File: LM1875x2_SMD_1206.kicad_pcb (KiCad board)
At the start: 2 copper layers, 27 parts, among them J1 INPUT, J2 OUTPUT, J3 POWER, U1 LM1875, U2 LM1875

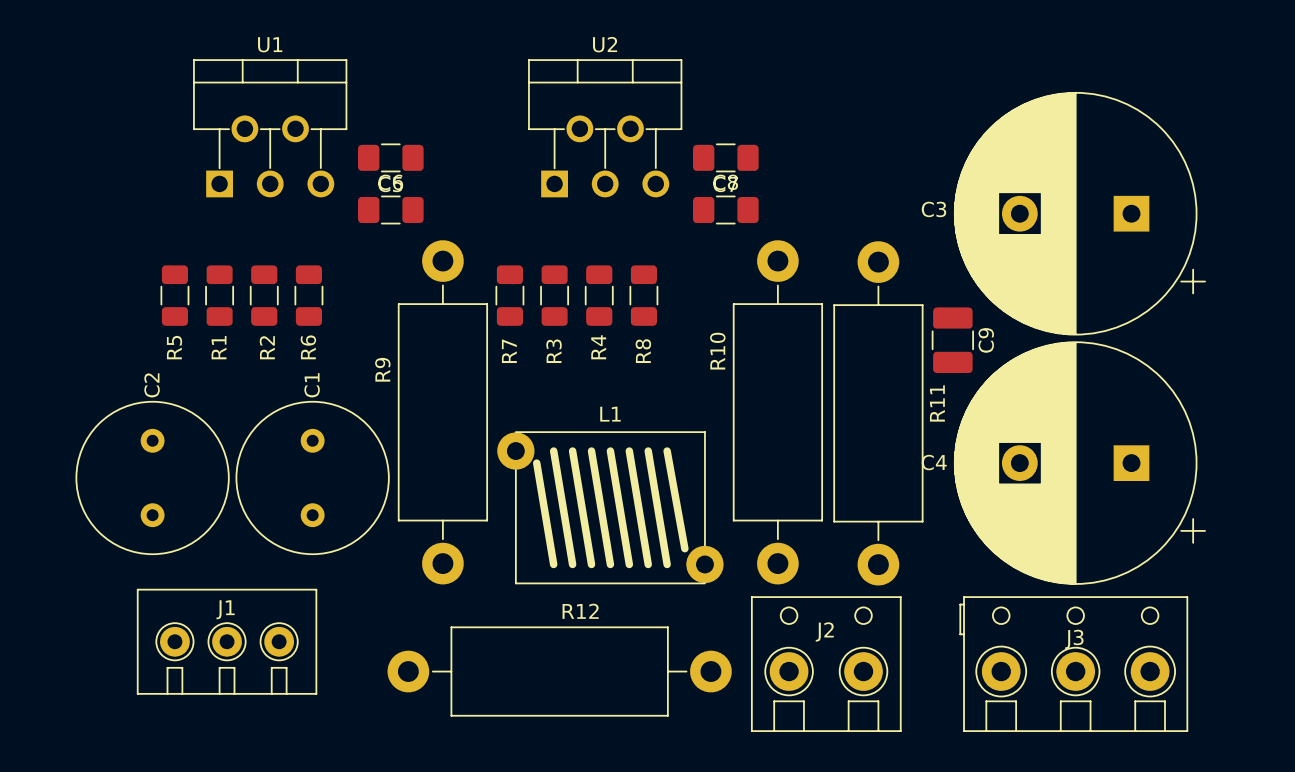
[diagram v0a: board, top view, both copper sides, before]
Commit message: finished layout
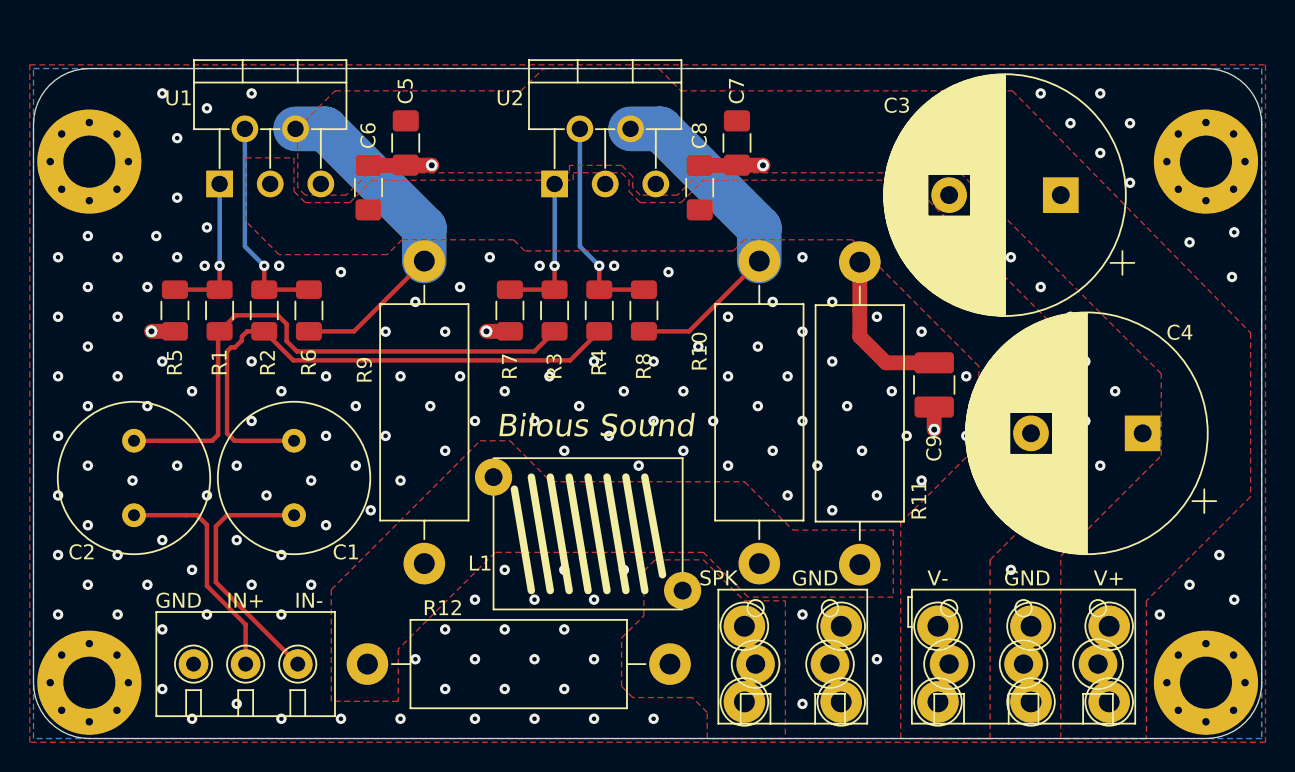
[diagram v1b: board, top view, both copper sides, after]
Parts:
- added H1: MountingHole, MountingHole:MountingHole_3.5mm_Pad_Via, F.Cu at (86.2, 88.8)
- added H2: MountingHole, MountingHole:MountingHole_3.5mm_Pad_Via, F.Cu at (86.2, 53.8)
- added H3: MountingHole, MountingHole:MountingHole_3.5mm_Pad_Via, F.Cu at (161.2, 53.8)
- added H4: MountingHole, MountingHole:MountingHole_3.5mm_Pad_Via, F.Cu at (161.2, 88.8)
- added J4: VCC, local_lib_footprints:Terminal_.25_PCB_TAB_TE_Connectivity_P5.08mm_, F.Cu at (154.8, 87.5)
- added J5: GND, local_lib_footprints:Terminal_.25_PCB_TAB_TE_Connectivity_P5.08mm_, F.Cu at (136.8, 87.5)
- added J6: VEE, local_lib_footprints:Terminal_.25_PCB_TAB_TE_Connectivity_P5.08mm_, F.Cu at (143.2, 87.5)
- added J7: SPK, local_lib_footprints:Terminal_.25_PCB_TAB_TE_Connectivity_P5.08mm_, F.Cu at (130.2, 87.5)
- added J8: GND, local_lib_footprints:Terminal_.25_PCB_TAB_TE_Connectivity_P5.08mm_, F.Cu at (149.5, 87.5)
- moved C3 4.91 mm to (151.5, 56.0)
- moved J3 3.54 mm to (149.0, 87.5)
- moved C9 3.25 mm to (143.0, 68.8)
- moved R12 2.80 mm to (125.2, 87.5)
- moved J2 2.30 mm to (133.5, 87.5)
- moved C8 2.30 mm to (127.2, 55.5), turned to 90 degrees
- moved L1 2.30 mm to (119.8, 78.8)
- moved C4 2.14 mm to (157.0, 72.0)
- moved C6 2.12 mm to (105.0, 55.5), turned to 90 degrees
- moved J1 1.95 mm to (96.8, 87.5)
- moved C5 1.41 mm to (107.5, 52.5), turned to 90 degrees
- moved C1 1.25 mm to (100.0, 72.5)
- moved C2 1.25 mm to (89.2, 72.5)
- moved C7 1.25 mm to (129.8, 52.5), turned to 90 degrees
- moved R10 1.25 mm to (131.2, 80.8)
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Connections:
- net Net-(J2-Pad1) renamed SPK
- net Net-(L1-Pad1) renamed /OUT
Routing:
- net Net-(C2-Pad1): track 0.00 -> 38.0 mm
- net Net-(C1-Pad1): track 0.00 -> 37.5 mm
- net Net-(R6-Pad1): track 0.00 -> 23.3 mm
- net Net-(R10-Pad2): track 0.00 -> 23.3 mm
- net Net-(C1-Pad2): track 0.00 -> 17.1 mm
- net Net-(C2-Pad2): track 0.00 -> 15.6 mm
- net Net-(R4-Pad1): track 0.00 -> 14.3 mm, vias 0 -> 1
- net Net-(R2-Pad1): track 0.00 -> 14.3 mm, vias 0 -> 1
- net GND: track 0.00 -> 13.2 mm, vias 0 -> 173
- net Net-(C9-Pad1): track 0.00 -> 10.7 mm
- net Net-(R3-Pad1): track 0.00 -> 10.1 mm, vias 0 -> 1
- net Net-(R1-Pad1): track 0.00 -> 10.1 mm, vias 0 -> 1
- added copper zone on F.Cu, net /OUT
- added copper zone on B.Cu, net GND
- added copper zone on F.Cu, net GND
- added copper zone on F.Cu, net SPK
- added copper zone on F.Cu, net VCC
- added copper zone on F.Cu, net VEE
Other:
- board outline added: 82.5 x 45 mm
- board text added: "Bilous Sound"
- board text added: "GND"
- board text added: "IN+"
- board text added: "IN-"
- board text added: "May 2023"
- board text added: "Rev 1.0"
- board text added: "SPK"
- board text added: "V+"
- board text added: "V-"
